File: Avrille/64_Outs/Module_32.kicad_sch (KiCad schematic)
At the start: 9 parts, among them J8 DIN41612_02x32_AC, U6 74HC595, U7 74HC595, U8 74HC595, U9 74HC595

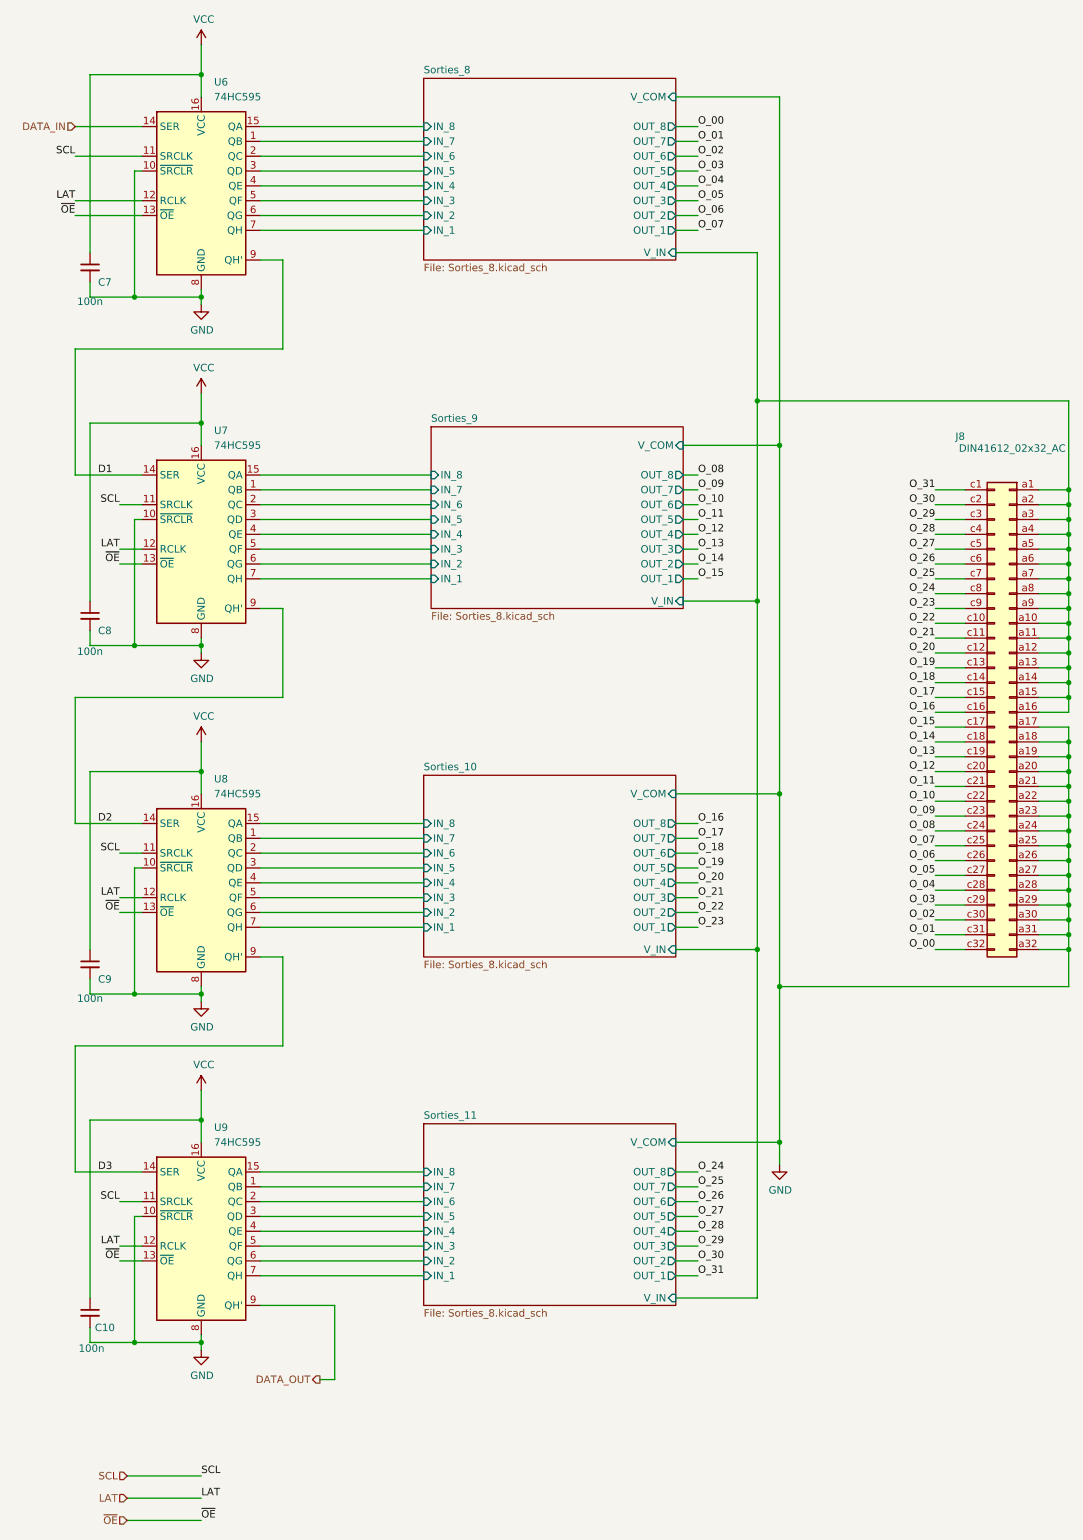
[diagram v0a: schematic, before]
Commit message: reset
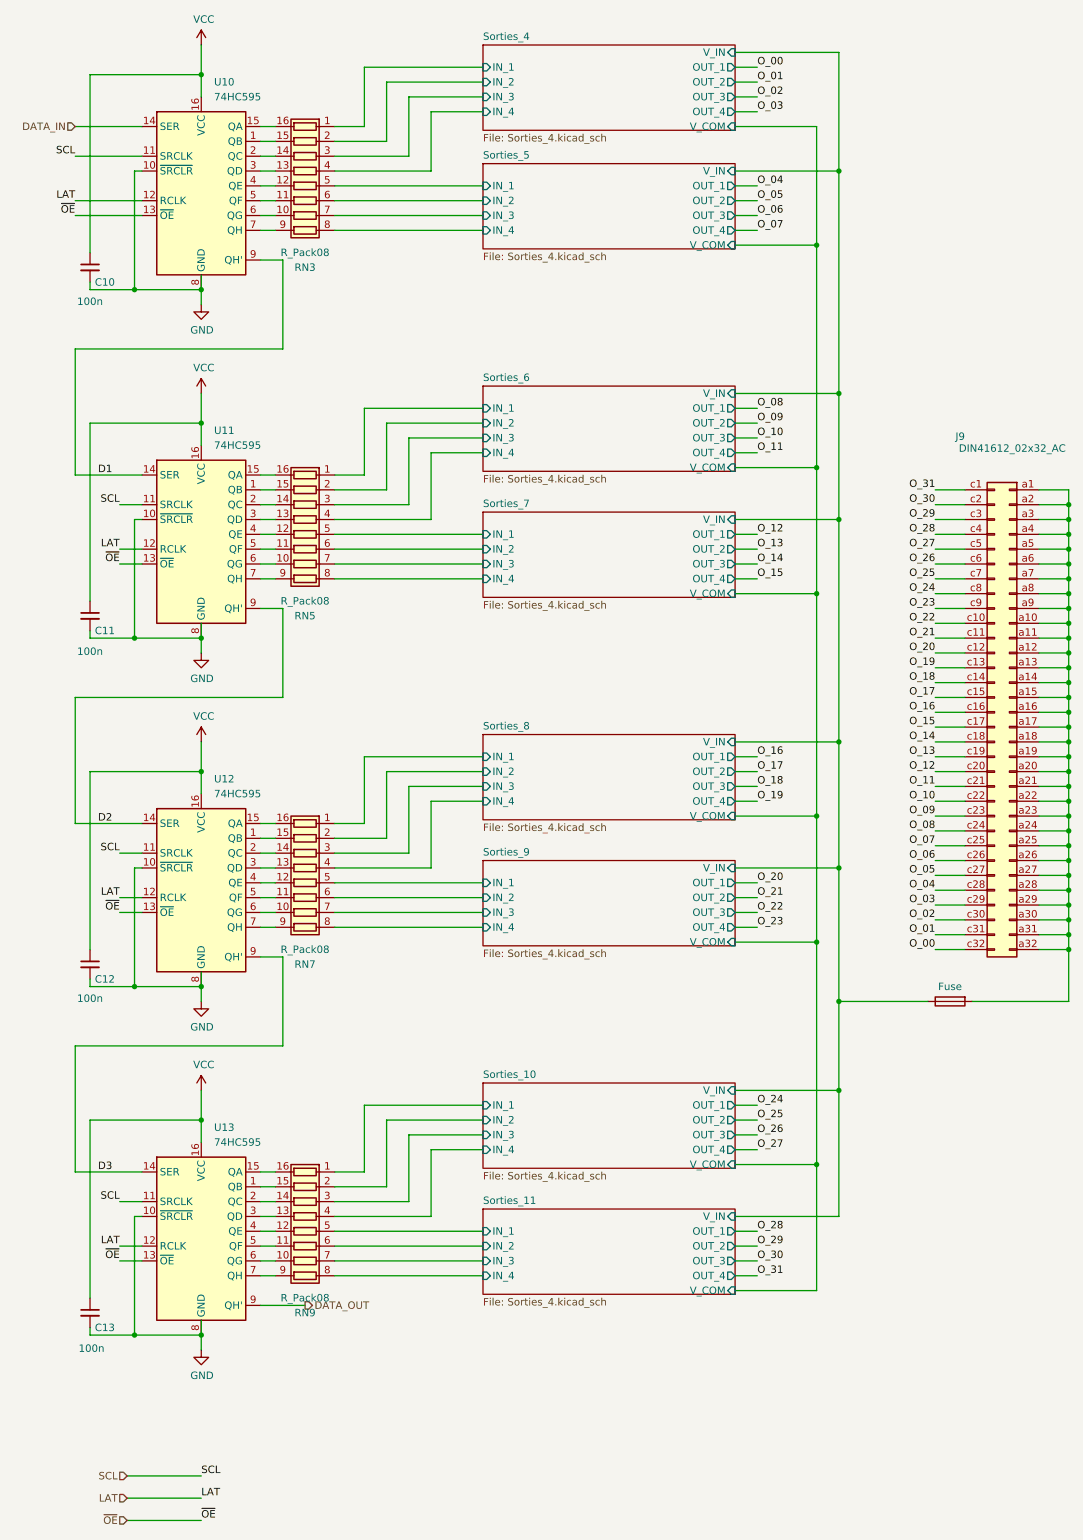
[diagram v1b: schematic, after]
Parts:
- added F3: Fuse, Fuse:Fuseholder_Clip-5x20mm_Bel_FC-203-22_Lateral_P17.80x5.00mm_D1.17mm_Horizontal, symbol Device:Fuse
- added RN3, RN5, RN7, RN9: R_Pack08, Package_DIP:DIP-16_W7.62mm, symbol Device:R_Pack08
- C10: renamed from C7; footprint Capacitor_THT:C_Disc_D5.0mm_W2.5mm_P2.50mm -> Capacitor_THT:C_Disc_D4.3mm_W1.9mm_P5.00mm
- C11: renamed from C8; footprint Capacitor_THT:C_Disc_D5.0mm_W2.5mm_P2.50mm -> Capacitor_THT:C_Disc_D4.3mm_W1.9mm_P5.00mm
- C12: renamed from C9; footprint Capacitor_THT:C_Disc_D5.0mm_W2.5mm_P2.50mm -> Capacitor_THT:C_Disc_D4.3mm_W1.9mm_P5.00mm
- C13: renamed from C10; footprint Capacitor_THT:C_Disc_D5.0mm_W2.5mm_P2.50mm -> Capacitor_THT:C_Disc_D4.3mm_W1.9mm_P5.00mm
- U10: renamed from U6; footprint Package_SO:SOIC-16W_7.5x12.8mm_P1.27mm -> Package_DIP:CERDIP-16_W7.62mm_SideBrazed
- U11: renamed from U7; footprint Package_SO:SOIC-16W_7.5x12.8mm_P1.27mm -> Package_DIP:CERDIP-16_W7.62mm_SideBrazed
- U12: renamed from U8; footprint Package_SO:SOIC-16W_7.5x12.8mm_P1.27mm -> Package_DIP:CERDIP-16_W7.62mm_SideBrazed
- U13: renamed from U9; footprint Package_SO:SOIC-16W_7.5x12.8mm_P1.27mm -> Package_DIP:CERDIP-16_W7.62mm_SideBrazed
- renumbered J8 to J9
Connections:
- net GND: no longer J9.a17 (Pin_a17), J9.a18 (Pin_a18), J9.a19 (Pin_a19), J9.a20 (Pin_a20), J9.a21 (Pin_a21), J9.a22 (Pin_a22), J9.a23 (Pin_a23), J9.a24 (Pin_a24), J9.a25 (Pin_a25), J9.a26 (Pin_a26), J9.a27 (Pin_a27), J9.a28 (Pin_a28), J9.a29 (Pin_a29), J9.a30 (Pin_a30), J9.a31 (Pin_a31), J9.a32 (Pin_a32)
- net Sorties_10/IN_1: now also RN9.1 (R1.1); no longer U12.7 (QH)
- net Sorties_10/IN_2: now also RN9.2 (R2.1); no longer U12.6 (QG)
- net Sorties_10/IN_3: now also RN9.3 (R3.1); no longer U12.5 (QF)
- net Sorties_10/IN_4: now also RN9.4 (R4.1); no longer U12.4 (QE)
- net Sorties_10/V_IN: now also F3.1; no longer J9.a1 (Pin_a1), J9.a10 (Pin_a10), J9.a11 (Pin_a11), J9.a12 (Pin_a12), J9.a13 (Pin_a13), J9.a14 (Pin_a14), J9.a15 (Pin_a15), J9.a16 (Pin_a16), J9.a2 (Pin_a2), J9.a3 (Pin_a3), J9.a4 (Pin_a4), J9.a5 (Pin_a5), J9.a6 (Pin_a6), J9.a7 (Pin_a7), J9.a8 (Pin_a8), J9.a9 (Pin_a9)
- net Sorties_11/IN_1: now also RN9.5 (R5.1); no longer U13.7 (QH)
- net Sorties_11/IN_2: now also RN9.6 (R6.1); no longer U13.6 (QG)
- net Sorties_11/IN_3: now also RN9.7 (R7.1); no longer U13.5 (QF)
- net Sorties_11/IN_4: now also RN9.8 (R8.1); no longer U13.4 (QE)
- net Sorties_8/IN_1: now also RN7.1 (R1.1); no longer U10.7 (QH)
- net Sorties_8/IN_2: now also RN7.2 (R2.1); no longer U10.6 (QG)
- net Sorties_8/IN_3: now also RN7.3 (R3.1); no longer U10.5 (QF)
- net Sorties_8/IN_4: now also RN7.4 (R4.1); no longer U10.4 (QE)
- net Sorties_9/IN_1: now also RN7.5 (R5.1); no longer U11.7 (QH)
- net Sorties_9/IN_2: now also RN7.6 (R6.1); no longer U11.6 (QG)
- net Sorties_9/IN_3: now also RN7.7 (R7.1); no longer U11.5 (QF)
- net Sorties_9/IN_4: now also RN7.8 (R8.1); no longer U11.4 (QE)
- net Sorties_10/IN_5: no longer names the net of U12.3 (QD)
- net Sorties_10/IN_5: now also RN7.13 (R4.2)
- net Sorties_10/IN_6: no longer names the net of U12.2 (QC)
- net Sorties_10/IN_6: now also RN7.14 (R3.2)
- net Sorties_10/IN_7: no longer names the net of U12.1 (QB)
- net Sorties_10/IN_7: now also RN7.15 (R2.2)
- net Sorties_10/IN_8: no longer names the net of U12.15 (QA)
- net Sorties_10/IN_8: now also RN7.16 (R1.2)
- net Sorties_11/IN_5: no longer names the net of U13.3 (QD)
- net Sorties_11/IN_5: now also RN9.13 (R4.2)
- net Sorties_11/IN_6: no longer names the net of U13.2 (QC)
- net Sorties_11/IN_6: now also RN9.14 (R3.2)
- net Sorties_11/IN_7: no longer names the net of U13.1 (QB)
- net Sorties_11/IN_7: now also RN9.15 (R2.2)
- net Sorties_11/IN_8: no longer names the net of U13.15 (QA)
- net Sorties_11/IN_8: now also RN9.16 (R1.2)
- net Sorties_8/IN_5: no longer names the net of U10.3 (QD)
- net Sorties_8/IN_5: now also RN3.13 (R4.2)
- net Sorties_8/IN_6: no longer names the net of U10.2 (QC)
- net Sorties_8/IN_6: now also RN3.14 (R3.2)
- net Sorties_8/IN_7: no longer names the net of U10.1 (QB)
- net Sorties_8/IN_7: now also RN3.15 (R2.2)
- net Sorties_8/IN_8: no longer names the net of U10.15 (QA)
- net Sorties_8/IN_8: now also RN3.16 (R1.2)
- net Sorties_9/IN_5: no longer names the net of U11.3 (QD)
- net Sorties_9/IN_5: now also RN5.13 (R4.2)
- net Sorties_9/IN_6: no longer names the net of U11.2 (QC)
- net Sorties_9/IN_6: now also RN5.14 (R3.2)
- net Sorties_9/IN_7: no longer names the net of U11.1 (QB)
- net Sorties_9/IN_7: now also RN5.15 (R2.2)
- net Sorties_9/IN_8: no longer names the net of U11.15 (QA)
- net Sorties_9/IN_8: now also RN5.16 (R1.2)
- new net: RN7.12 (R5.2), U12.4 (QE)
- new net: RN7.11 (R6.2), U12.5 (QF)
- new net: RN7.10 (R7.2), U12.6 (QG)
- new net: RN7.9 (R8.2), U12.7 (QH)
- new net: RN3.12 (R5.2), U10.4 (QE)
- new net: RN3.11 (R6.2), U10.5 (QF)
- new net: RN3.10 (R7.2), U10.6 (QG)
- new net: RN3.9 (R8.2), U10.7 (QH)
- new net: RN9.12 (R5.2), U13.4 (QE)
- new net: RN9.11 (R6.2), U13.5 (QF)
- new net: RN9.10 (R7.2), U13.6 (QG)
- new net: RN9.9 (R8.2), U13.7 (QH)
- new net: RN5.10 (R7.2), U11.6 (QG)
- new net: RN5.11 (R6.2), U11.5 (QF)
- new net: RN5.12 (R5.2), U11.4 (QE)
- new net: RN5.9 (R8.2), U11.7 (QH)
- new net: F3.2, J9.a1 (Pin_a1), J9.a10 (Pin_a10), J9.a11 (Pin_a11), J9.a12 (Pin_a12), J9.a13 (Pin_a13), J9.a14 (Pin_a14), J9.a15 (Pin_a15), J9.a16 (Pin_a16), J9.a17 (Pin_a17), J9.a18 (Pin_a18), J9.a19 (Pin_a19), J9.a2 (Pin_a2), J9.a20 (Pin_a20), J9.a21 (Pin_a21), J9.a22 (Pin_a22), J9.a23 (Pin_a23), J9.a24 (Pin_a24), J9.a25 (Pin_a25), J9.a26 (Pin_a26), J9.a27 (Pin_a27), J9.a28 (Pin_a28), J9.a29 (Pin_a29), J9.a3 (Pin_a3), J9.a30 (Pin_a30), J9.a31 (Pin_a31), J9.a32 (Pin_a32), J9.a4 (Pin_a4), J9.a5 (Pin_a5), J9.a6 (Pin_a6), J9.a7 (Pin_a7), J9.a8 (Pin_a8), J9.a9 (Pin_a9)
- new net Sorties_4/IN_1: RN3.1 (R1.1)
- new net Sorties_4/IN_2: RN3.2 (R2.1)
- new net Sorties_4/IN_3: RN3.3 (R3.1)
- new net Sorties_4/IN_4: RN3.4 (R4.1)
- new net Sorties_5/IN_1: RN3.5 (R5.1)
- new net Sorties_5/IN_2: RN3.6 (R6.1)
- new net Sorties_5/IN_3: RN3.7 (R7.1)
- new net Sorties_5/IN_4: RN3.8 (R8.1)
- new net Sorties_6/IN_1: RN5.1 (R1.1)
- new net Sorties_6/IN_2: RN5.2 (R2.1)
- new net Sorties_6/IN_3: RN5.3 (R3.1)
- new net Sorties_6/IN_4: RN5.4 (R4.1)
- new net Sorties_7/IN_1: RN5.5 (R5.1)
- new net Sorties_7/IN_2: RN5.6 (R6.1)
- new net Sorties_7/IN_3: RN5.7 (R7.1)
- new net Sorties_7/IN_4: RN5.8 (R8.1)
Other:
- added sheet Sorties_4 (Sorties_4.kicad_sch)
- added sheet Sorties_5 (Sorties_4.kicad_sch)
- added sheet Sorties_6 (Sorties_4.kicad_sch)
- added sheet Sorties_7 (Sorties_4.kicad_sch)
- sheet Sorties_10: file Sorties_8.kicad_sch -> Sorties_4.kicad_sch
- sheet Sorties_10 ports: added none; removed IN_5, IN_6, IN_7, IN_8, OUT_5, OUT_6, OUT_7, OUT_8
- sheet Sorties_11: file Sorties_8.kicad_sch -> Sorties_4.kicad_sch
- sheet Sorties_11 ports: added none; removed IN_5, IN_6, IN_7, IN_8, OUT_5, OUT_6, OUT_7, OUT_8
- sheet Sorties_8: file Sorties_8.kicad_sch -> Sorties_4.kicad_sch
- sheet Sorties_8 ports: added none; removed IN_5, IN_6, IN_7, IN_8, OUT_5, OUT_6, OUT_7, OUT_8
- sheet Sorties_9: file Sorties_8.kicad_sch -> Sorties_4.kicad_sch
- sheet Sorties_9 ports: added none; removed IN_5, IN_6, IN_7, IN_8, OUT_5, OUT_6, OUT_7, OUT_8
- title: Carte Midi - 64 Sorties -> Module SPI - 32 Sorties
